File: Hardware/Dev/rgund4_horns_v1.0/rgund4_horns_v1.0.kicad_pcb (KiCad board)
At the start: 2 copper layers, 44.5 x 28.5 mm, 23 parts, among them J1 24V Battery, J2 Horn_Control, J3 Horn_out_Upper, J4 Horn_out_Lower, Q1 IRFR010PBF, SW1 BUTTON

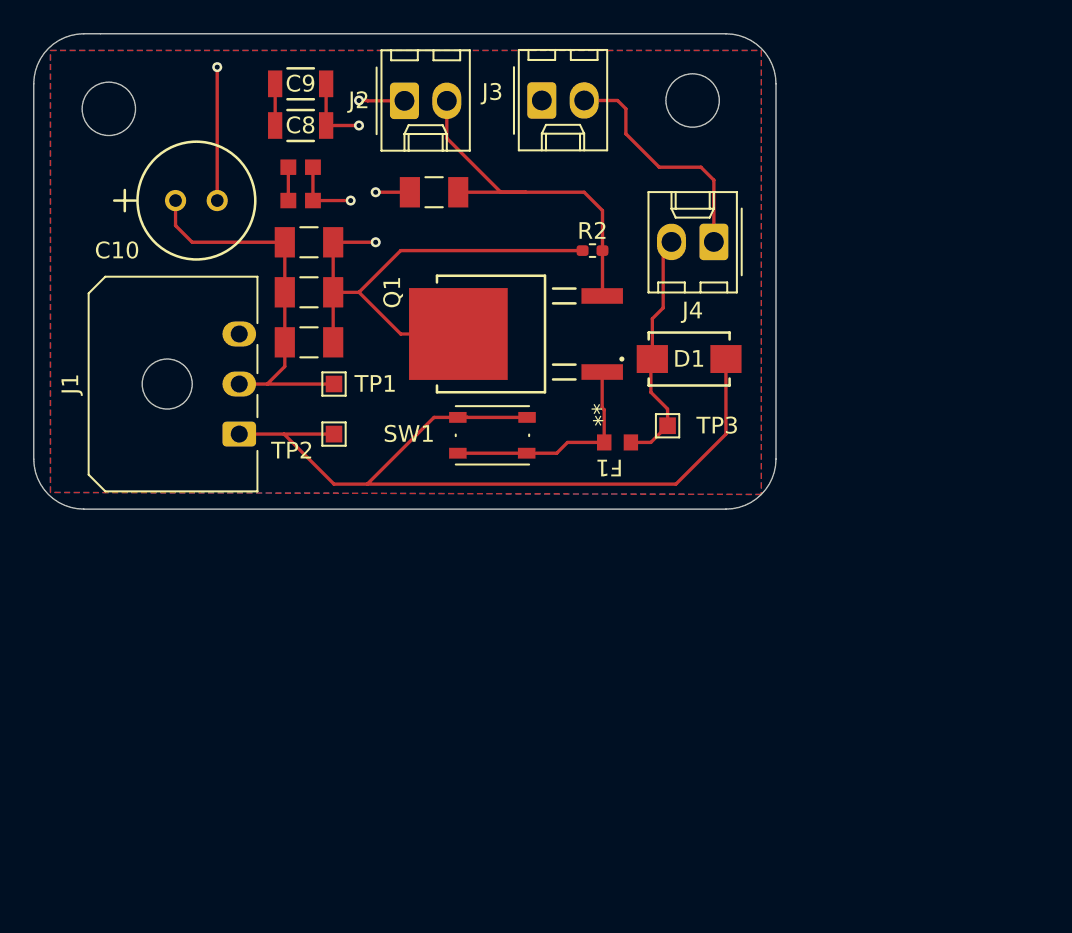
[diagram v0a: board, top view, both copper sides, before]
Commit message: finished finished
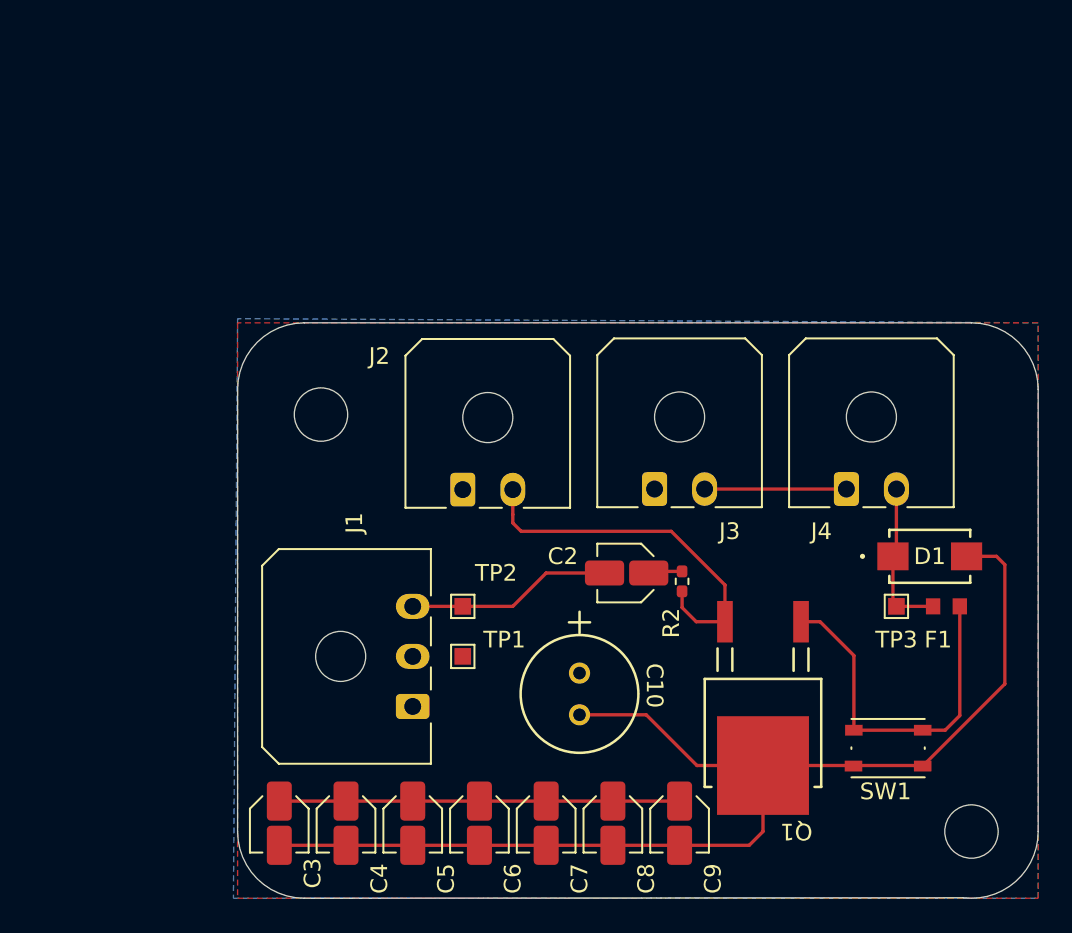
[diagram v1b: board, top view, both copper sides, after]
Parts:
- removed the REF** at (143.5, 72.0)
- removed the REF** at (108.5, 72.5)
- added REF**: MountingHole_3.2mm_M3, MountingHole:MountingHole_3.2mm_M3, F.Cu at (121.2, 90.8)
- added REF**: MountingHole_3.2mm_M3, MountingHole:MountingHole_3.2mm_M3, F.Cu at (160.2, 115.8)
- C2, C3, C4, C5: footprint Specfic footprints:CAPC3216X180N -> Capacitor_SMD:C_Elec_3x5.4
- C6, C7: footprint Specfic footprints:CAPC1608X90N(1uF) -> Capacitor_SMD:C_Elec_3x5.4
- C8, C9: footprint Specfic footprints:CAP_CL31_SAM(10uF) -> Capacitor_SMD:C_Elec_3x5.4
- J2, J3, J4: footprint Connector_Molex:Molex_KK-254_AE-6410-02A_1x02_P2.54mm_Vertical -> Connector_Molex:Molex_Micro-Fit_3.0_43650-0200_1x02_P3.00mm_Horizontal
- moved C9 49.8 mm to (142.7, 115.3), turned to -90 degrees
- moved C8 45.8 mm to (138.7, 115.3), turned to -90 degrees
- moved C7 42.0 mm to (134.7, 115.3), turned to -90 degrees
- moved C6 38.8 mm to (130.7, 115.3), turned to -90 degrees
- moved C10 37.3 mm to (136.7, 106.3), turned to -90 degrees
- moved C3 34.9 mm to (118.7, 115.3), turned to -90 degrees
- moved C4 31.9 mm to (122.7, 115.3), turned to -90 degrees
- moved SW1 30.2 mm to (155.2, 110.8), turned to 180 degrees
- moved C5 29.5 mm to (126.7, 115.3), turned to -90 degrees
- moved Q1 28.9 mm to (147.7, 109.9), turned to 180 degrees
- moved C2 25.6 mm to (139.5, 100.3)
- moved J3 24.3 mm to (141.2, 95.3)
- moved J2 23.6 mm to (129.7, 95.3)
- moved F1 22.0 mm to (158.7, 102.3), turned to 0 degrees
- moved R2 20.5 mm to (142.9, 100.8), turned to -90 degrees
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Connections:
- C2 pad 1: /Control -> Net-(C2-Pad1)
- R2 pad 1: GND -> Net-(C2-Pad1)
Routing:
- net GND: track 104.5 -> 84.1 mm, vias 6 -> 0
- net /High : track 13.3 -> 21.7 mm
- net Net-(J3-Pin_2): track 14.3 -> 8.50 mm
- net /HORN_IN: track 14.4 -> 9.11 mm
- net +24V: track 27.6 -> 24.0 mm
- net Net-(C2-Pad1): track 0.00 -> 2.04 mm
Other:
- board size 44.5 x 28.5 mm -> 48 x 34.5 mm
